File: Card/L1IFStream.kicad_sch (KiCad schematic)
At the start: 107 parts, among them J1 Conn_Coaxial, J2 USB_A, J3 RF_Shield_One_Piece, J4 Conn_Coaxial, U1 MAX2769ETI+T, U10 74LVC374, U11 74HC2GU04, U2 TPS717285DCKR, U3 TPS717285DCKR, U4 NCP164CSN330T1G, U5 93LC66BT-I_OT, U6 FT2232H-Interface_USB, U7 74LVC1G74, U8 74LVC1G04, U9 74LVC374, X1 SIT5156, X2 SIT2024BA-S8-33E-12.00000E, X3 QPQ1060

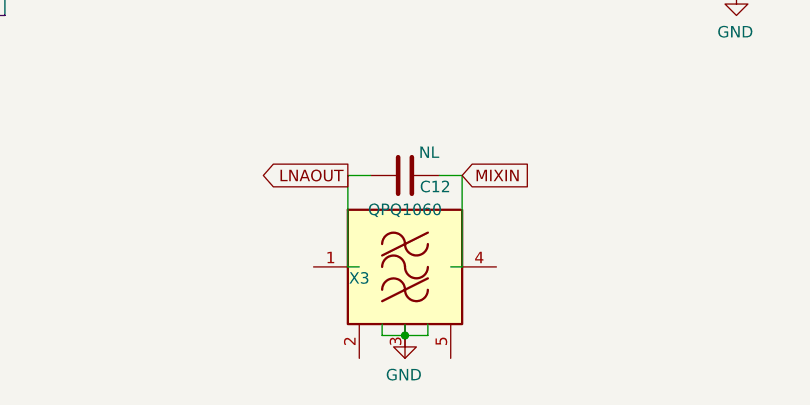
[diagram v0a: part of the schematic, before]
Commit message: Sent parts to PCBway
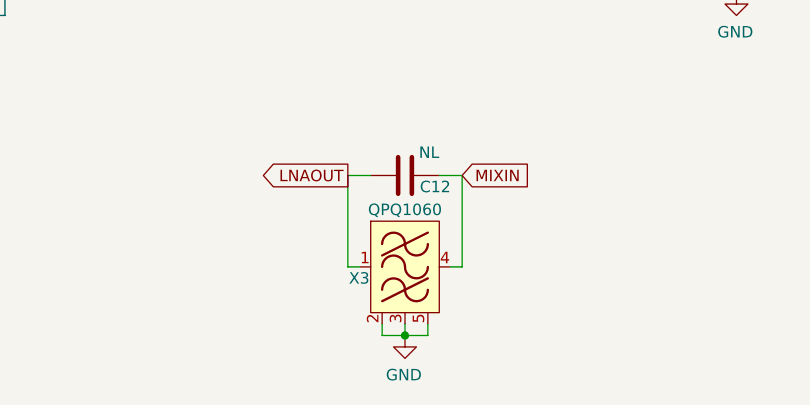
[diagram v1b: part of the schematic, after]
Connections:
- net GND: now also X3.2 (GND), X3.3 (GND), X3.5 (GND)
- net LNAOUT: now also X3.1 (IN)
- net MIXIN: now also X3.4 (OUT)
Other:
- moved on the sheet: X3
